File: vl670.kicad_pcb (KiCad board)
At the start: 4 copper layers, 64.9 x 25.1 mm, 106 parts, among them J1 Conn_01x07_Male, J2 USB_C_Receptacle, J3 Conn_01x07_Male, J4 USB3_A Receptacle, J5 Conn_01x02_Male, U1 HD3SS3220, U2 VL670, U3 74LVC2G66, U4 TPS2061C-PXLI, U5 74LVC2G66, U6 GD25D05, Y1 25MHz

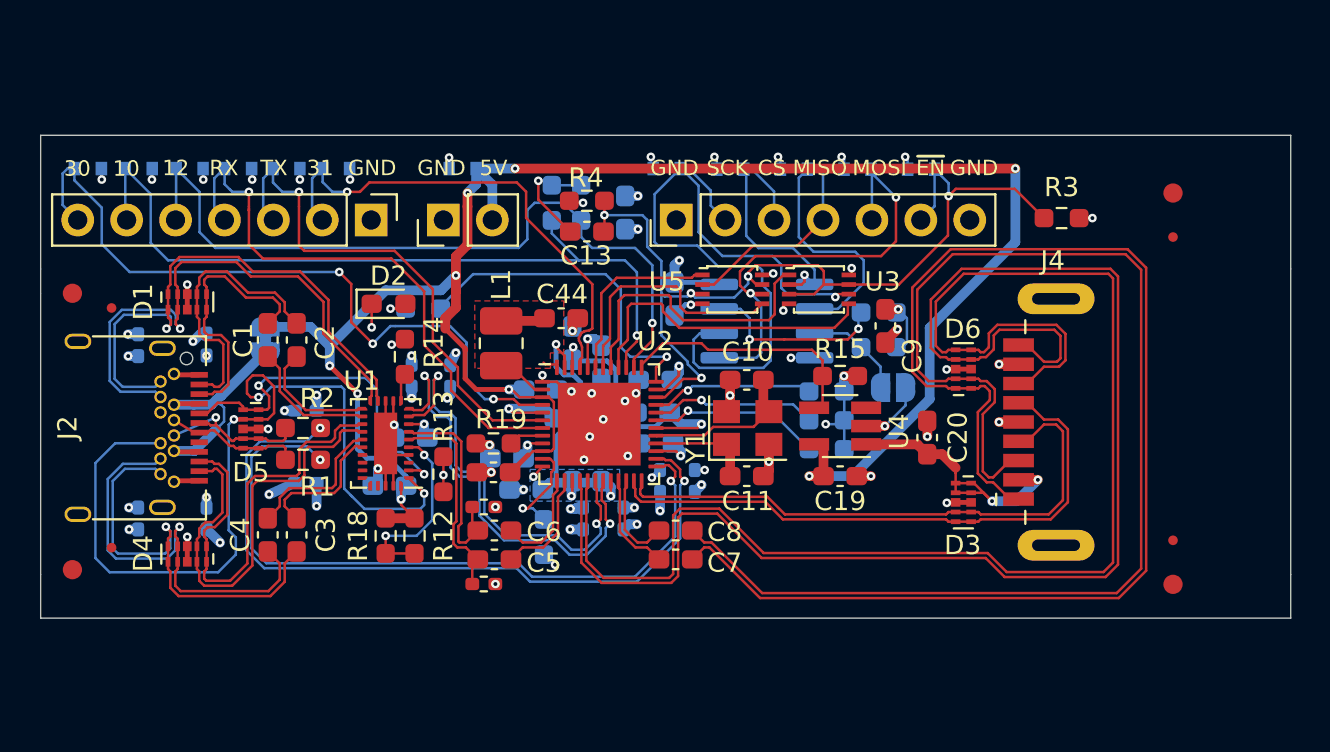
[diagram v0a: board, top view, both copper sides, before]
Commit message: v0.02.
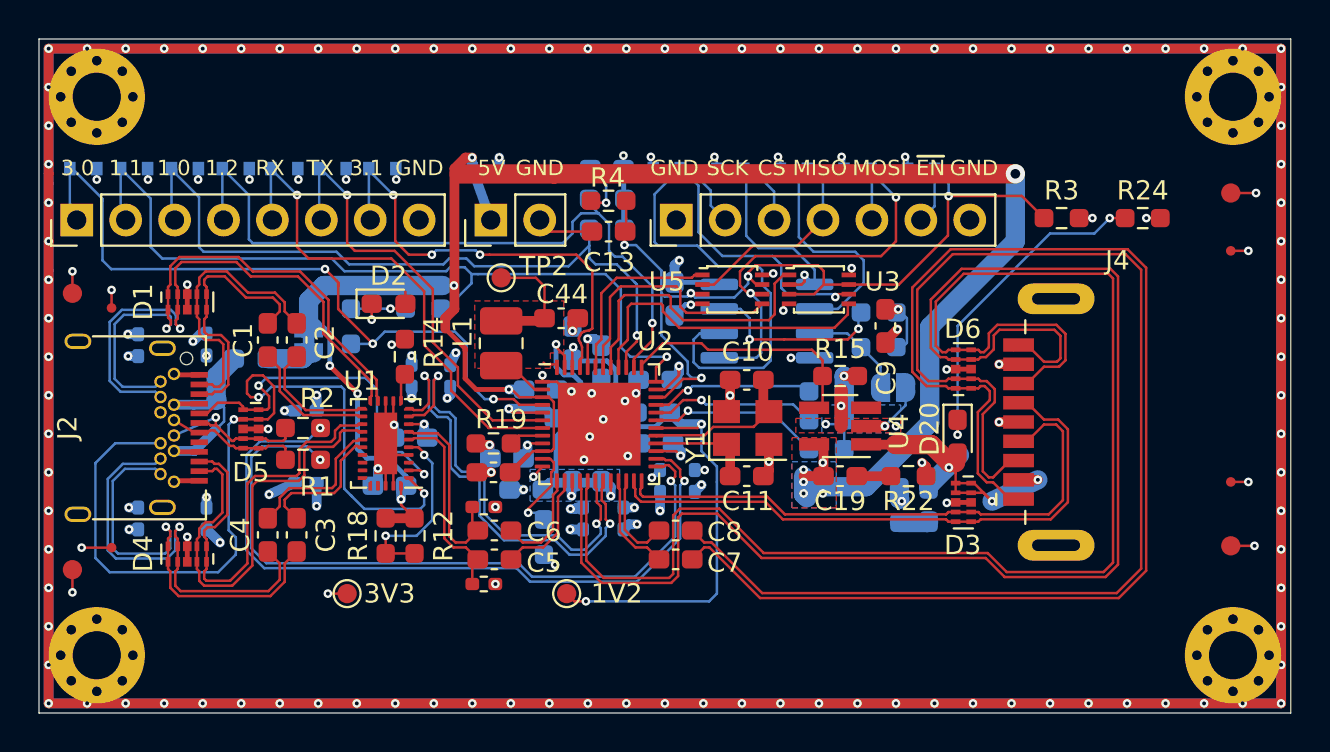
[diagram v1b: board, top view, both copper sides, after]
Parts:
- added D19: ESD7951S, Diode_SMD:D_SOD-523, B.Cu at (174.3, 109.7)
- added D20: LED, LED_SMD:LED_0603_1608Metric_Pad1.05x0.95mm_HandSolder, F.Cu at (219.7, 123.7)
- added FB1: Ferrite_Bead_Small, Inductor_SMD:L_0603_1608Metric_Pad1.05x0.95mm_HandSolder, B.Cu at (183.0, 119.6)
- added H1: MountingHole_Pad, MountingHole:MountingHole_2.5mm_Pad_Via, F.Cu at (175.0, 106.0)
- added H2: MountingHole_Pad, MountingHole:MountingHole_2.5mm_Pad_Via, F.Cu at (175.0, 135.0)
- added H3: MountingHole_Pad, MountingHole:MountingHole_2.5mm_Pad_Via, F.Cu at (234.0, 106.0)
- added H4: MountingHole_Pad, MountingHole:MountingHole_2.5mm_Pad_Via, F.Cu at (234.0, 135.0)
- added R22: 0R5, Resistor_SMD:R_0603_1608Metric_Pad0.98x0.95mm_HandSolder, F.Cu at (217.2, 125.7)
- added R23: 0R5, Resistor_SMD:R_0603_1608Metric_Pad0.98x0.95mm_HandSolder, B.Cu at (216.7, 127.2)
- added R24: 470R, Resistor_SMD:R_0603_1608Metric_Pad0.98x0.95mm_HandSolder, F.Cu at (229.3, 112.3)
- added TP1: TestPoint, TestPoint:TestPoint_Pad_D1.0mm, F.Cu at (188.0, 131.8)
- added TP2: TestPoint, TestPoint:TestPoint_Pad_D1.0mm, F.Cu at (196.0, 115.4)
- added TP3: TestPoint, TestPoint:TestPoint_Pad_D1.0mm, F.Cu at (199.4, 131.8)
- C10, C11: value 20pF -> 18pF
- C19: value 1uF -> 10uF
- C20: value 1uF -> 10uF; moved to B.Cu
- C7, C8: value 100nF -> 220nF
- J3: value Conn_01x07_Male -> Conn_01x08_Male; footprint Connector_PinHeader_2.54mm:PinHeader_1x07_P2.54mm_Vertical -> Connector_PinHeader_2.54mm:PinHeader_1x08_P2.54mm_Vertical
- R13: value NC -> 470R; moved to B.Cu
- moved J3 15.3 mm to (174.0, 112.4), turned to 90 degrees
- moved R13 9.06 mm to (188.2, 117.9)
- moved FID8 4.27 mm to (233.9, 126.0)
- moved FID7 3.61 mm to (233.9, 129.3)
- moved C20 3.50 mm to (218.2, 127.2), turned to 270 degrees
- moved R21 3.16 mm to (201.5, 112.9), turned to 0 degrees
- moved FID6 3.08 mm to (233.9, 114.0)
- moved FID3 3.00 mm to (233.9, 111.0)
- moved J5 2.46 mm to (195.5, 112.4)
- moved C22 2.46 mm to (201.5, 109.8), turned to 0 degrees
- moved D10 2.40 mm to (184.7, 109.7)
- moved D11 2.40 mm to (187.2, 109.7)
- moved D12 2.40 mm to (189.8, 109.7)
- moved D7 2.40 mm to (176.9, 109.7)
- moved D8 2.40 mm to (179.6, 109.7)
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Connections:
- C19 pad 2: GND -> Net-(C19-Pad2)
- C20 pad 2: GND -> Net-(C20-Pad2)
- FID1 pad : (no net) -> GND
- FID2 pad : (no net) -> GND
- FID3 pad : (no net) -> GND
- FID4 pad : (no net) -> GND
- FID5 pad : (no net) -> GND
- FID6 pad : (no net) -> GND
- FID7 pad : (no net) -> GND
- FID8 pad : (no net) -> GND
- J3 pad 1: GND -> Net-(D19-Pad1)
- J3 pad 2: Net-(D12-Pad1) -> Net-(D7-Pad1)
- J3 pad 3: Net-(D11-Pad1) -> Net-(D8-Pad1)
- J3 pad 4: Net-(D10-Pad1) -> Net-(D9-Pad1)
- J3 pad 5: Net-(D9-Pad1) -> Net-(D10-Pad1)
- J3 pad 6: Net-(D8-Pad1) -> Net-(D11-Pad1)
- J3 pad 7: Net-(D7-Pad1) -> Net-(D12-Pad1)
- J5 pad 1: GND -> +5V
- J5 pad 2: +5V -> GND
- JP2 pad 1: +5VP -> Net-(FB1-Pad1)
- R13 pad 1: GND -> Net-(D2-Pad2)
- R13 pad 2: GND -> Net-(D19-Pad1)
- R9 pad 2: Net-(R9-Pad2) -> Net-(D7-Pad1)
- U2 pad 36: Net-(R9-Pad2) -> Net-(D7-Pad1)
- U2 pad 4: Net-(D7-Pad1) -> Net-(D19-Pad1)
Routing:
- net GND: track 85.5 -> 686.8 mm, vias 64 -> 172
- net Net-(D19-Pad1): track 0.00 -> 38.7 mm, vias 0 -> 3
- net Net-(R9-Pad2): track 17.7 -> 0.00 mm, vias 1 -> 0
- net Net-(D20-Pad1): track 0.00 -> 17.4 mm, vias 0 -> 2
- net +1V2: track 15.1 -> 32.3 mm, vias 2 -> 3
- net +5V: track 105.1 -> 112.7 mm, vias 9 -> 12
- net Net-(D7-Pad1): track 37.9 -> 43.5 mm, vias 3 -> 1
- net +1V5: track 21.3 -> 25.4 mm
- net Net-(D8-Pad1): track 41.3 -> 38.3 mm
- net Net-(D2-Pad2): track 1.67 -> 4.43 mm
- net Net-(D10-Pad1): track 30.0 -> 27.4 mm
- net Net-(D11-Pad1): track 27.1 -> 24.5 mm
- net Net-(FB1-Pad1): track 0.00 -> 2.25 mm
- net Net-(D12-Pad1): track 26.5 -> 24.3 mm, vias 1 -> 3
- net +3V3: track 35.2 -> 37.4 mm
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- added copper zone on B.Cu, net +5V
- added copper zone on F.Cu, net +5V
- added copper zone on B.Cu, net GND
- added copper zone on F.Cu, net GND
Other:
- board size 64.9 x 25.1 mm -> 65 x 35 mm
- board text added: "1.0"
- board text added: "1.1"
- board text added: "1.2"
- board text added: "3.0"
- board text added: "3.1"
- board text added: "VL670"
- board text added: "VL671"
- board text removed: "10"
- board text removed: "12"
- board text removed: "30"
- board text removed: "31"
